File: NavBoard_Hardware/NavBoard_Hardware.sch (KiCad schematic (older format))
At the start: 59 parts, among them J1 Conn_Coaxial, Q1 BSS138, Q2 BSS138, U2 ATMEGA328P-Project_Library, U3 OKI, U4 OKI, U5 FGPMMOPA6H, Y1 Crystal

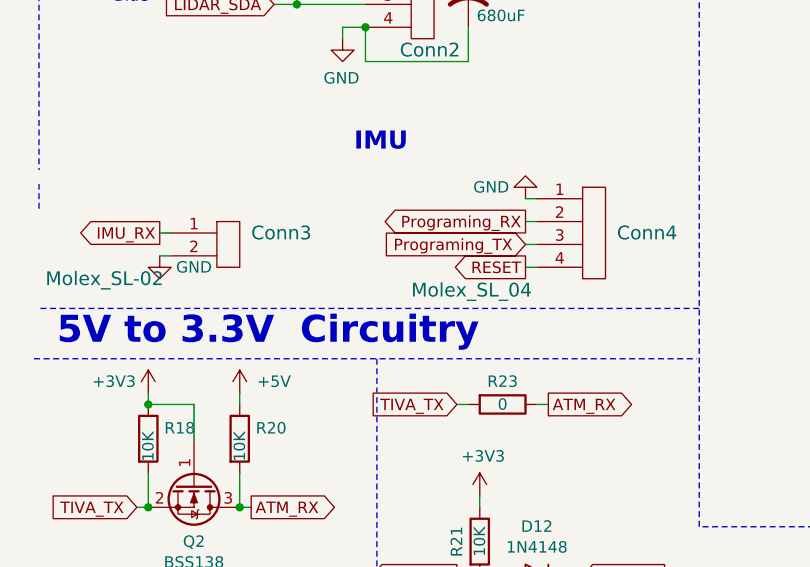
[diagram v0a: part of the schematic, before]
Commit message: REV 2
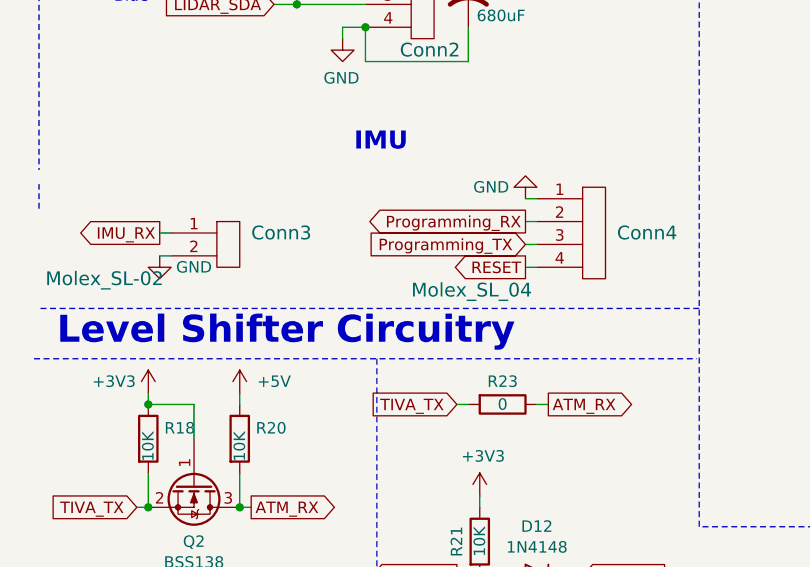
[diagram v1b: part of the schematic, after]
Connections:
- net Programing_RX is gone; now on net Programming_RX: Conn4.2
- net Programing_TX is gone; now on net Programming_TX: Conn4.3
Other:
- note added: "Level Shifter Circuitry"
- note removed: "5V to 3.3V Circuitry"
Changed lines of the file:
@@
 	1000 5250 1050 5250
 Text GLabel 2600 5200 0    50   Output ~ 0
-Programing_RX
+Programming_RX
 Text GLabel 2600 5300 0    50   Input ~ 0
-Programing_TX
+Programming_TX
 Text GLabel 2600 5400 0    50   Output ~ 0
 RESET
@@
 add 15K resistor in place\nof diode to create a voltage divider.\n
 Text Notes 550  5750 0    118  ~ 24
-5V to 3.3V  Circuitry
+Level Shifter Circuitry
 Wire Notes Line
 	450  5800 3350 5800

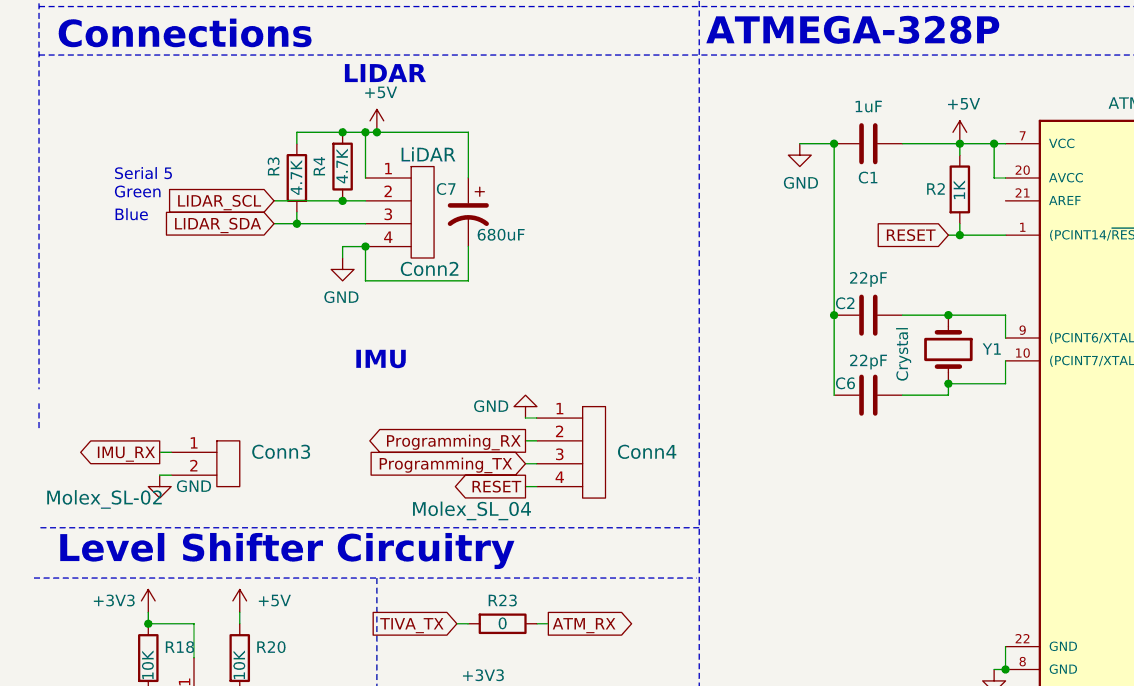
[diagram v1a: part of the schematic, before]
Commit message: Final touches
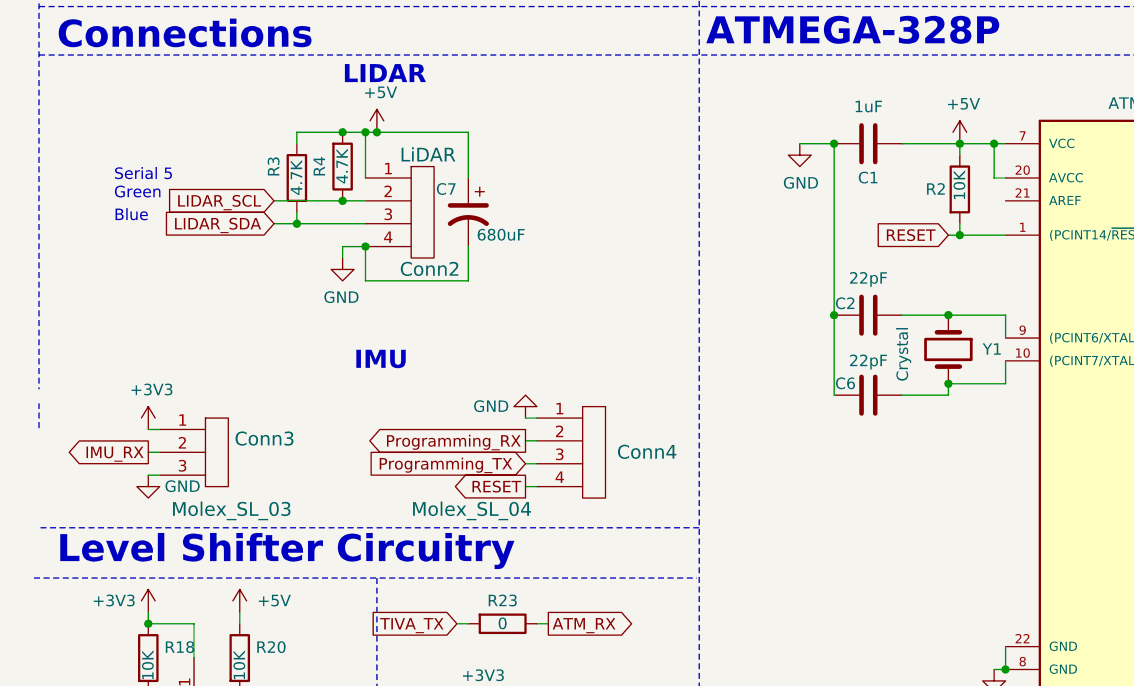
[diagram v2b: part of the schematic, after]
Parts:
- removed Conn3: Molex_SL-02, MRDT_Connectors:MOLEX_SL_02_Horizontal, symbol NavBoard_Hardware-rescue:Molex_SL_02-MRDT_Connectors
- added Conn3: Molex_SL_03, MRDT_Connectors:MOLEX_SL_03_Horizontal, symbol NavBoard_Hardware-rescue:Molex_SL_03-MRDT_Connectors
- R2: value 1K -> 10K
- U2: footprint (none) -> Package_DIP:DIP-28_W7.62mm
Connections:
- net +3V3: now also Conn3.1
- net GND: now also Conn3.3
- net IMU_RX: now also Conn3.2
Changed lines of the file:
@@
 F 0 "U2" H 5650 8967 50  0000 C CNN
 F 1 "ATMEGA328P-Project_Library" H 5650 8876 50  0000 C CNN
-F 2 "" H 5600 7600 50  0001 C CIN
+F 2 "Package_DIP:DIP-28_W7.62mm" H 5600 7600 50  0001 C CIN
 F 3 "" H 5600 7600 50  0001 C CNN
 	1    4850 6300
@@
 P 4500 4100
 F 0 "R2" H 4350 4100 50  0000 L CNN
-F 1 "1K" V 4500 4050 50  0000 L CNN
+F 1 "10K" V 4500 4050 50  0000 L CNN
 F 2 "Resistor_SMD:R_0603_1608Metric_Pad1.05x0.95mm_HandSolder" V 4430 4100 50  0001 C CNN
 F 3 "~" H 4500 4100 50  0001 C CNN
@@
 	10800 4800 10800 4850
 $Comp
-L NavBoard_Hardware-rescue:Molex_SL_02-MRDT_Connectors Conn3
-U 1 1 5C7D6386
-P 1250 5400
-F 0 "Conn3" H 1400 5550 60  0000 L CNN
-F 1 "Molex_SL-02" H 500 5350 60  0000 L CNN
-F 2 "MRDT_Connectors:MOLEX_SL_02_Horizontal" H 1250 5400 60  0001 C CNN
-F 3 "" H 1250 5400 60  0001 C CNN
-	1    1250 5400
-	1    0    0    -1
-$EndComp
-$Comp
 L NavBoard_Hardware-rescue:Molex_SL_04-MRDT_Connectors Conn4
 U 1 1 5C7FFA12
@@
 	1    0    0    -1
 $EndComp
-Text GLabel 1000 5250 0    50   Output ~ 0
+Text GLabel 950  5250 0    50   Output ~ 0
 IMU_RX
 Wire Wire Line
-	1000 5250 1050 5250
+	950  5250 1000 5250
 Text GLabel 2600 5200 0    50   Output ~ 0
 Programming_RX
@@
 L power:GND #PWR0127
 U 1 1 5C819482
-P 1000 5350
-F 0 "#PWR0127" H 1000 5100 50  0001 C CNN
-F 1 "GND" H 1150 5300 50  0000 C CNN
-F 2 "" H 1000 5350 50  0001 C CNN
-F 3 "" H 1000 5350 50  0001 C CNN
-	1    1000 5350
+P 950 5350
+F 0 "#PWR0127" H 950 5100 50  0001 C CNN
+F 1 "GND" H 1100 5300 50  0000 C CNN
+F 2 "" H 950 5350 50  0001 C CNN
+F 3 "" H 950 5350 50  0001 C CNN
+	1    950  5350
 	1    0    0    -1
 $EndComp
@@
 	4000 6550 4000 7800
 Wire Wire Line
-	1050 5350 1000 5350
+	1000 5350 950  5350
 Text Notes 7350 7500 0    91   ~ 0
 Navigation PCB Rev. 2\n
@@
 Text Notes 10600 7650 0    50   ~ 0
 2\n
+$Comp
+L NavBoard_Hardware-rescue:Molex_SL_03-MRDT_Connectors Conn3
+U 1 1 5C7DBB4B
+P 1200 5400
+F 0 "Conn3" H 1327 5608 60  0000 L CNN
+F 1 "Molex_SL_03" H 1050 5300 60  0000 L CNN
+F 2 "MRDT_Connectors:MOLEX_SL_03_Horizontal" H 1200 5400 60  0001 C CNN
+F 3 "" H 1200 5400 60  0001 C CNN
+	1    1200 5400
+	1    0    0    -1
+$EndComp
+$Comp
+L power:+3V3 #PWR0129
+U 1 1 5C7F8FA0
+P 950 5150
+F 0 "#PWR0129" H 950 5000 50  0001 C CNN
+F 1 "+3V3" H 965 5323 50  0000 C CNN
+F 2 "" H 950 5150 50  0001 C CNN
+F 3 "" H 950 5150 50  0001 C CNN
+	1    950  5150
+	1    0    0    -1
+$EndComp
+Wire Wire Line
+	1000 5150 950  5150
 $EndSCHEMATC
